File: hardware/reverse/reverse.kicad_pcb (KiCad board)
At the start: 2 copper layers, 50 x 50 mm, 55 parts, among them J1 Conn_01x03, U1 CH32V003F4U6

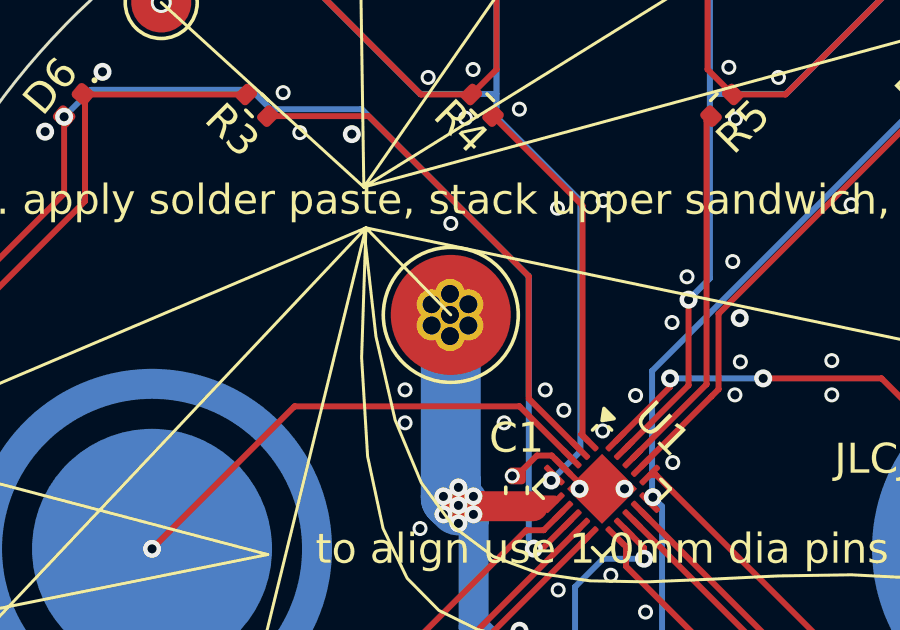
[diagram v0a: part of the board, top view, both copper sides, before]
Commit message: update fab files
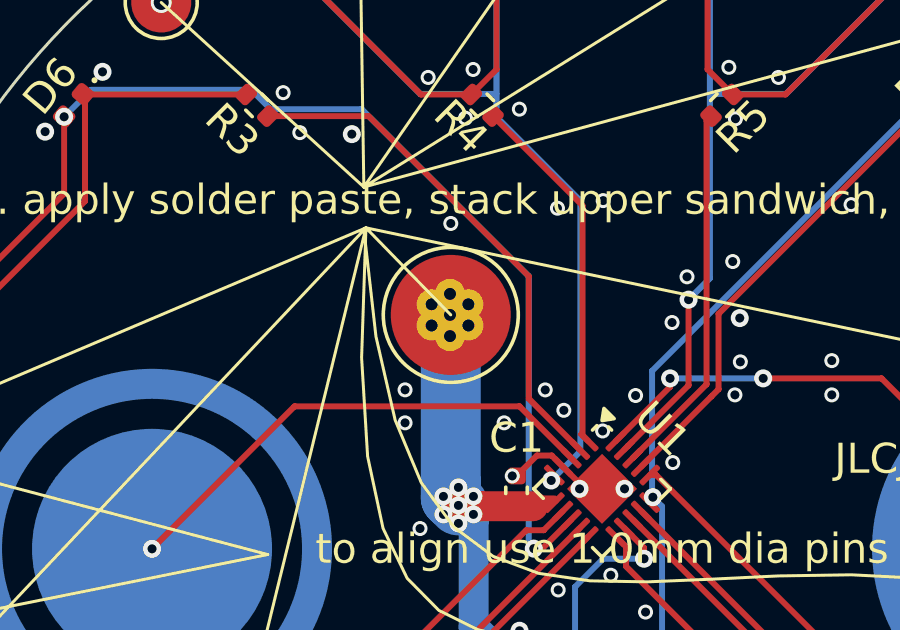
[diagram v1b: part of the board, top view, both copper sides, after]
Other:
- board text removed: "import QR SVG scale 0.2"
- board text removed: "import rear (Inkscape) SVG scale 0.075"
